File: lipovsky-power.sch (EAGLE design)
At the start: 98 parts, among them J1 M04-929J, J2 M04-929J, J3 M04-929J, J4 M04-929J, Q1 NMOS30V_30A, Q12 NMOS40V_10A, Q14 NMOS40V_10A, Q16 NMOS40V_10A, Q18 NMOS40V_10A, Q21 PMOS30V_11A, Q22 PMOS30V_11A, Q23 NMOS40V_10A, Q24 NMOS40V_10A, Q25 PMOS30V_11A, Q26 PMOS30V_11A, Q27 NMOS40V_10A, Q28 NMOS40V_10A, Q3 2PMOS50V_0.17A, Q31 PMOS30V_11A, Q32 PMOS30V_11A, Q33 PMOS30V_11A, Q34 PMOS30V_11A, Q35 PMOS30V_11A, Q36 PMOS30V_11A, Q37 PMOS30V_11A, Q38 PMOS30V_11A, Q4 2PMOS50V_0.17A, Q41 PMOS30V_11A, Q42 PMOS30V_11A, Q43 PMOS30V_11A, Q44 PMOS30V_11A, Q45 PMOS30V_11A, Q46 PMOS30V_11A, Q47 PMOS30V_11A, Q48 PMOS30V_11A, Q5 2NMOS30V_0.1A, Q51 PMOS30V_11A, Q52 PMOS30V_11A, Q53 PMOS30V_11A, Q54 PMOS30V_11A, Q55 PMOS30V_11A, Q56 PMOS30V_11A, Q57 PMOS30V_11A, Q58 PMOS30V_11A, Q62 PMOS30V_11A, Q64 PMOS30V_11A, Q66 PMOS30V_11A, Q68 PMOS30V_11A, T1 TFORM_4_4311_4A4, U1 DG508BEN-T1-GE4, U2 DG508BEN-T1-GE4, U4 LTC3805-5IDD, U6 AR30N60PPA-13

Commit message: 2S boost
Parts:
- removed D4: D_ZENER2.4V, dubec:D_ZENER2.4V
- removed MVOE: ATTINYX4A2MMHR, dubec:ATTINYX4A2MMHR
- added CB1, CB2, CB3: CAP4.7UF_10V, dubec:CAP4.7UF_10V
- added D2: D_ZENER2.4V, dubec:D_ZENER2.4V
- added DB1: 2D_SCHOTTKY40V_0.2A, dubec:2D_SCHOTTKY40V_0.2A
- added U3: DG508BEN-T1-GE4, dubec:DG508BEN-T1-GE4
- added U5: LM2665M6, dubec:LM2665M6
- U1: value DG508BEN-T1-GE4 -> LTC3805-5IDD; device dubec:DG508BEN-T1-GE4 -> dubec:LTC3805-5IDD
- U2: value DG508BEN-T1-GE4 -> ATTINYX4A2MMHR; device dubec:DG508BEN-T1-GE4 -> dubec:ATTINYX4A2MMHR
- U4: value LTC3805-5IDD -> DG508BEN-T1-GE4; device dubec:LTC3805-5IDD -> dubec:DG508BEN-T1-GE4
- renumbered U$2 to JP2, U$3 to DA1, U$4 to DA2
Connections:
- new net 2SBOOST: CB3.2, DB1G$1.A, DB1G$2.C, U5.OUT
- new net N$11: CB2.1, U5.CAP-
- new net N$2: CB1.2, DB1G$2.A, U5.V+
- new net N$9: CB2.2, U5.CAP+
- net !GS1: now also U3.S1; no longer U1.S1
- net !GT1: now also U4.S2; no longer U2.S2
- net !S_RESET: now also U2.PB3; no longer MVOE.PB3
- net +5V: now also U2.VCC; no longer MVOE.VCC
- net +8V: now also U1.VCC; no longer U4.VCC
- net AS0: now also U2.PA2, U3.A0; no longer MVOE.PA2, U1.A0
- net AS1: now also U2.PA1, U3.A1; no longer MVOE.PA1, U1.A1
- net AS2: now also U2.PA0, U3.A2; no longer MVOE.PA0, U1.A2
- net AT0: now also U2.PB2, U4.A0; no longer MVOE.PB2, U2.A0
- net AT1: now also U2.PB1, U4.A1; no longer MVOE.PB1, U2.A1
- net AT2: now also U2.PB0, U4.A2; no longer MVOE.PB0, U2.A2
- net BATT+: now also U3.EN, U3.V+, U4.EN, U4.V+; no longer U1.EN, U1.V+, U2.EN, U2.V+
- net BATT-: now also U3.D, U3.S7, U3.S8, U3.V-, U4.D, U4.S1, U4.S8, U4.V-; no longer U1.D, U1.S7, U1.S8, U1.V-, U2.D, U2.S1, U2.S8, U2.V-
- net C1: now also CB3.1, U5.GND, U5.SD
- net C2: now also CB1.1
- net C4+: now also DB1G$1.C
- net EN_FLYBACK: now also U1.RUN, U2.PA3; no longer MVOE.PA3, U4.RUN
- net FB: now also U2.PA7; no longer MVOE.PA7
- net GS+2: now also U3.S2; no longer U1.S2
- net GS3: now also U3.S3; no longer U1.S3
- net GS4: now also U3.S4; no longer U1.S4
- net GS5: now also U3.S5; no longer U1.S5
- net GS6: now also U3.S6; no longer U1.S6
- net GT+2: now also U4.S3; no longer U2.S3
- net GT3: now also U4.S4; no longer U2.S4
- net GT4: now also U4.S5; no longer U2.S5
- net GT5: now also U4.S6; no longer U2.S6
- net GT6: now also U4.S7; no longer U2.S7
- net MISO: now also U2.PA5; no longer MVOE.PA5
- net N$1: now also D2.C, U1.FB; no longer D4.C, U4.FB
- net N$12: now also U1.I_TH; no longer U4.I_TH
- net N$3: now also U1.FS; no longer U4.FS
- net N$4: now also U1.OC; no longer U4.OC
- net N$5: now also U1.GATE; no longer U4.GATE
- net N$6: now also U1.I_SENSE; no longer U4.I_SENSE
- net S-: now also D2.A, U1.SYNC, U3.GND; no longer D4.A, MVOE.GND, U4.SYNC
- net SCL: now also U2.PA4; no longer MVOE.PA4
- net SDA: now also U2.PA6; no longer MVOE.PA6
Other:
- note added: "2S Booster"
- moved on the sheet: J1, J2, J3, J4, JP1, Q12, Q14, Q16, Q18, Q21, Q22, Q23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

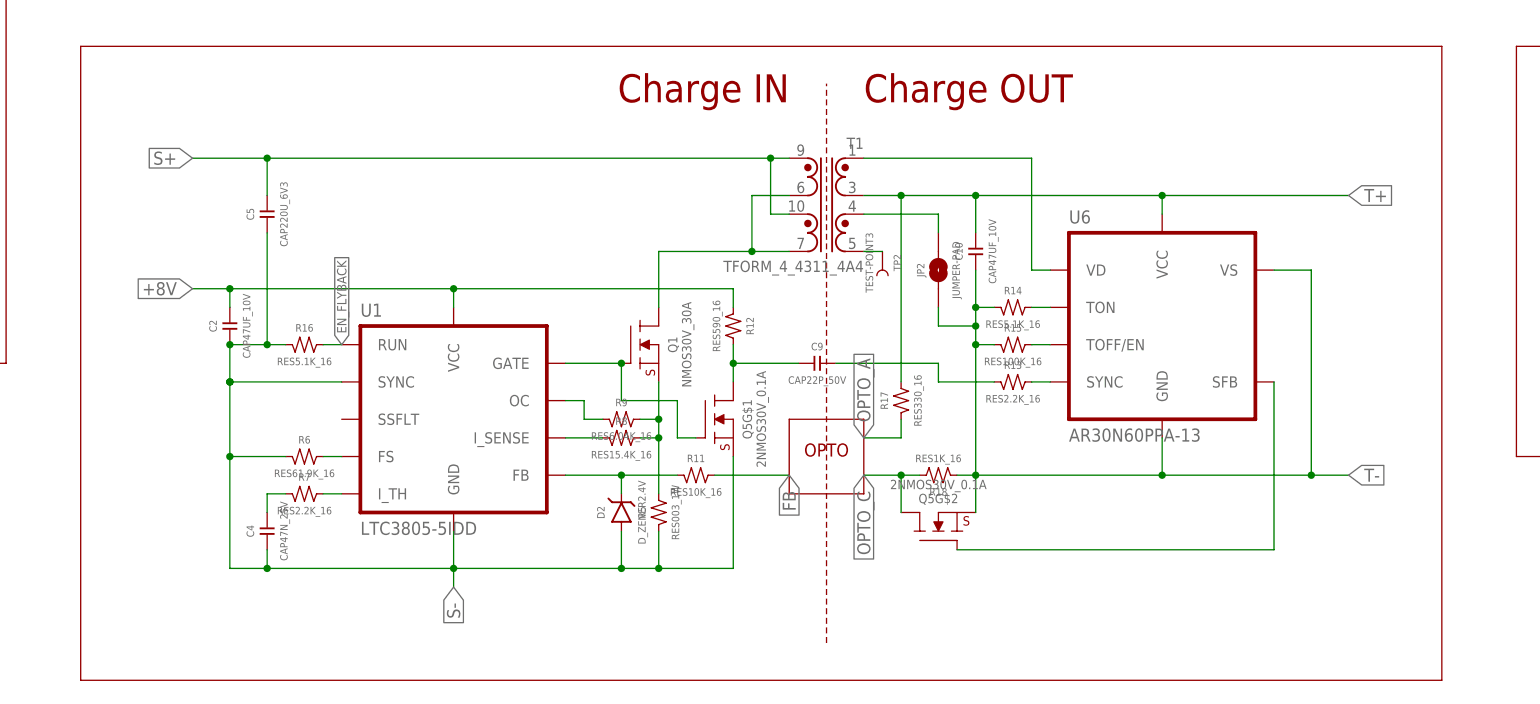
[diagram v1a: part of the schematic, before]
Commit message: Inductor routing
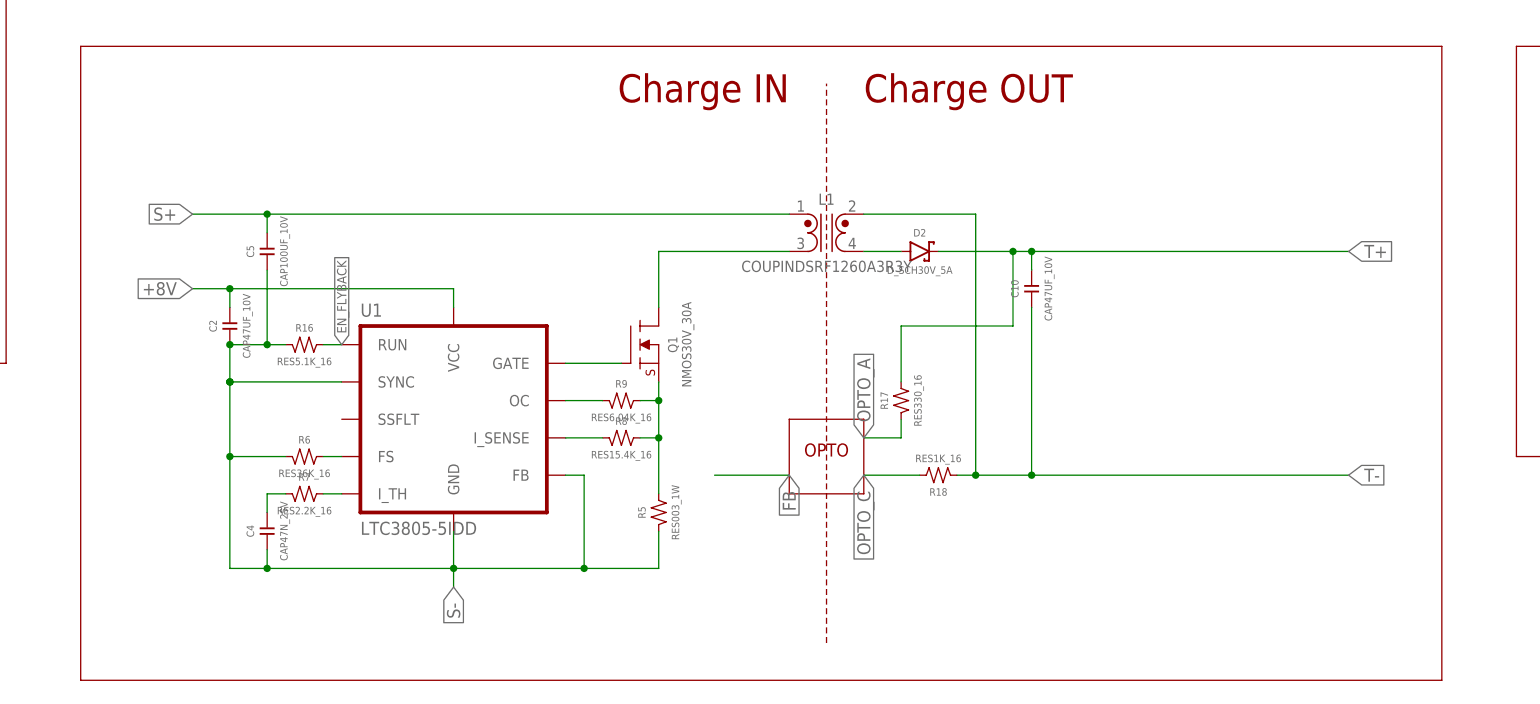
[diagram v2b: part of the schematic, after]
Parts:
- removed C9: CAP22P_50V, dubec:CAP22P_50V
- removed JP2: JUMPER-PAD, dubec:JUMPER-PAD
- removed Q5: 2NMOS30V_0.1A, dubec:2NMOS30V_0.1A
- removed R11: RES10K_16, dubec:RES10K_16
- removed R12: RES590_16, dubec:RES590_16
- removed R13: RES2.2K_16, dubec:RES2.2K_16
- removed R14: RES5.1K_16, dubec:RES5.1K_16
- removed R15: RES100K_16, dubec:RES100K_16
- removed T1: TFORM_4_4311_4A4, dubec:TFORM_4_4311_4A4
- removed TP2: TEST-POINT3, SparkFun-Passives:TEST-POINT3
- removed U6: AR30N60PPA-13, dubec:AR30N60PPA-13
- added L1: COUPINDSRF1260A3R3Y, dubec:COUPINDSRF1260A3R3Y
- C5: value CAP220U_6V3 -> CAP100UF_10V; device dubec:CAP220U_6V3 -> dubec:CAP100UF_10V
- D2: value D_ZENER2.4V -> D_SCH30V_5A; device dubec:D_ZENER2.4V -> dubec:D_SCH30V_5A
- R6: value RES61.9K_16 -> RES36K_16; device dubec:RES61.9K_16 -> dubec:RES36K_16
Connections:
- removed net N$1: D2.C, R11.1, U1.FB
- removed net N$18: C9.1, Q5G$1.D, R12.2
- removed net N$20: C9.2, R13.1
- removed net N$21: R13.2, U6.SYNC
- removed net N$24: R14.2, U6.TON
- removed net N$25: R15.2, U6.TOFF/EN
- removed net N$26: T1.1, U6.VD
- removed net N$8: T1.4, TP2.1
- removed net SFB: Q5G$2.G, U6.SFB
- net +8V: no longer R12.1
- net FB: no longer R11.2
- net N$10: now also L1.A2; no longer T1.5, T1.7
- net N$5: no longer Q5G$1.G
- net N$7: now also D2.A, L1.B2; no longer JP2.2, T1.3
- net OPTO_C: no longer Q5G$2.D
- net S+: now also L1.A1; no longer T1.6, T1.8
- net S-: now also U1.FB; no longer D2.A, Q5G$1.S
- net T+: now also D2.C; no longer T1.2, U6.VCC
- net T-: now also L1.B1; no longer JP2.1, Q5G$2.S, R14.1, R15.1, U6.GND, U6.VS
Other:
- moved on the sheet: C10, C5, R9

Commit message: "finished"
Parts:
- removed C4: CAP47N_25V, dubec:CAP47N_25V
- added D3: D_SCH30V_0.2A, dubec:D_SCH30V_0.2A
- R7: value RES2.2K_16 -> RES18.2K_16; device dubec:RES2.2K_16 -> dubec:RES18.2K_16
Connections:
- removed net N$12: R7.2, U1.I_TH
- removed net N$17: C4.2, R7.1
- new net N$1: D3.A, U1.I_TH
- new net TH: D3.C, R7.1
- net +8V: now also R7.2
- net S-: no longer C4.1
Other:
- moved on the sheet: C10, CB1, CB2, CB3, D2, DB1G$2, J1, J2, J3, J4, JP1, L1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
